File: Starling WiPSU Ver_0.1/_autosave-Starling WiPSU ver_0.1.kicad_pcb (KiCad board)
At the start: 2 copper layers, 60 x 19.5 mm, 26 parts, among them CON1 9V/2A, P1 HC-05 Bluetooth, P2 ESP8266 - 01, P3 CONN_01X01, P4 CONN_01X01, P6 2.3" Display Conn, Q1 BSS138, Q2 BSS138, Q3 BC847, SW1 SW_PUSH, U1 LM317S, U2 1117-3.3

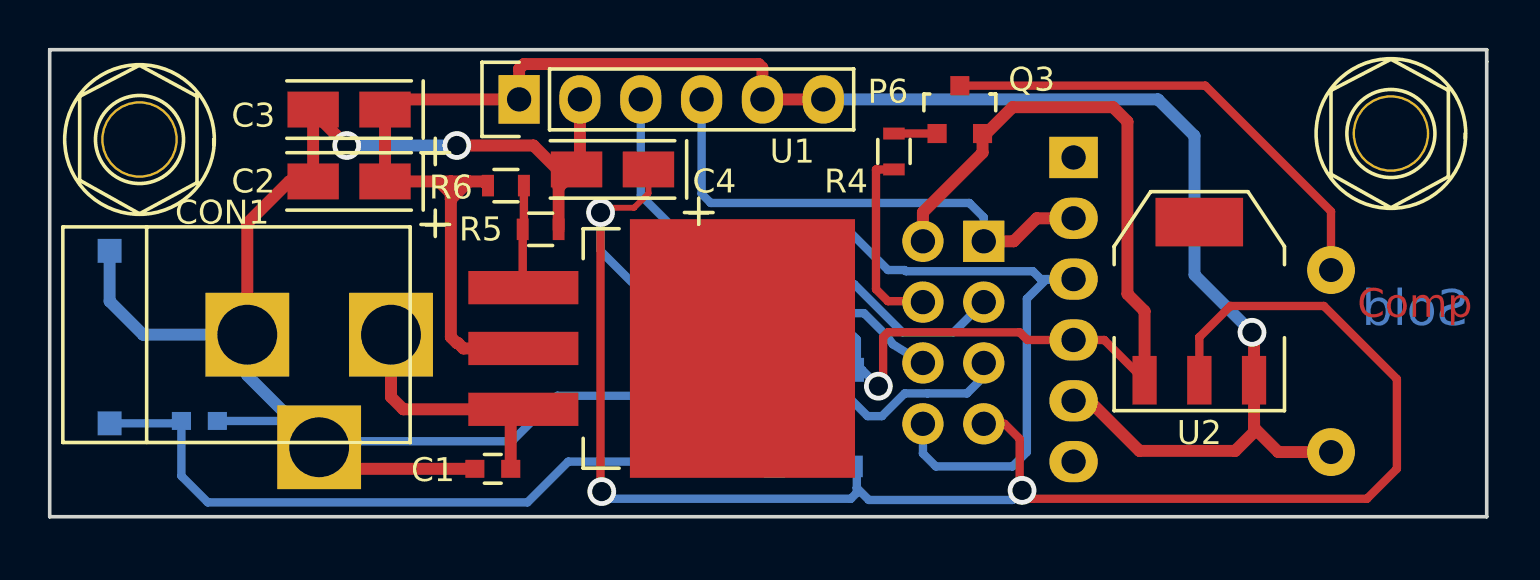
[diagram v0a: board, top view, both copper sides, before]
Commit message: Wifi and PSU ver0.1 updated
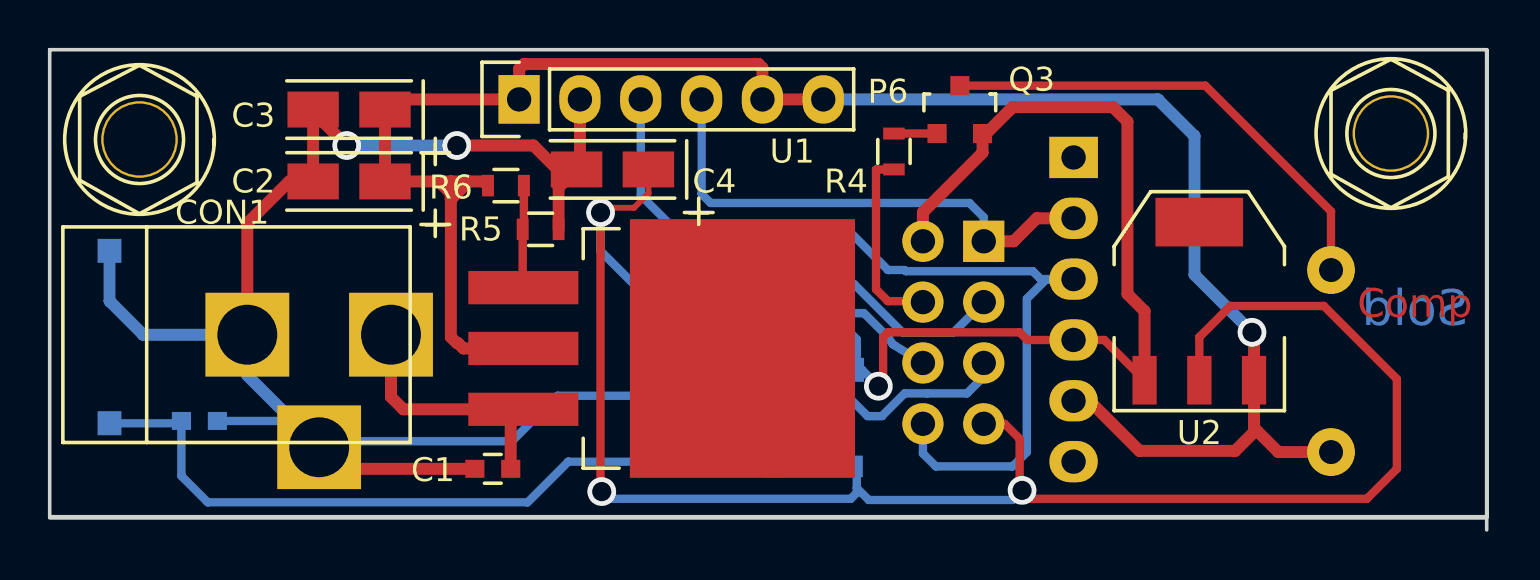
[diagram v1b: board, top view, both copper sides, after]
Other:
- board size 60 x 19.5 mm -> 60 x 20 mm
